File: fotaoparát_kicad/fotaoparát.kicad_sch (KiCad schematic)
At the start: 5 parts, among them IC1 W25Q256JVEIQ, J2 Micro_SD_Card_Det1, U2 CR2013-MI2120

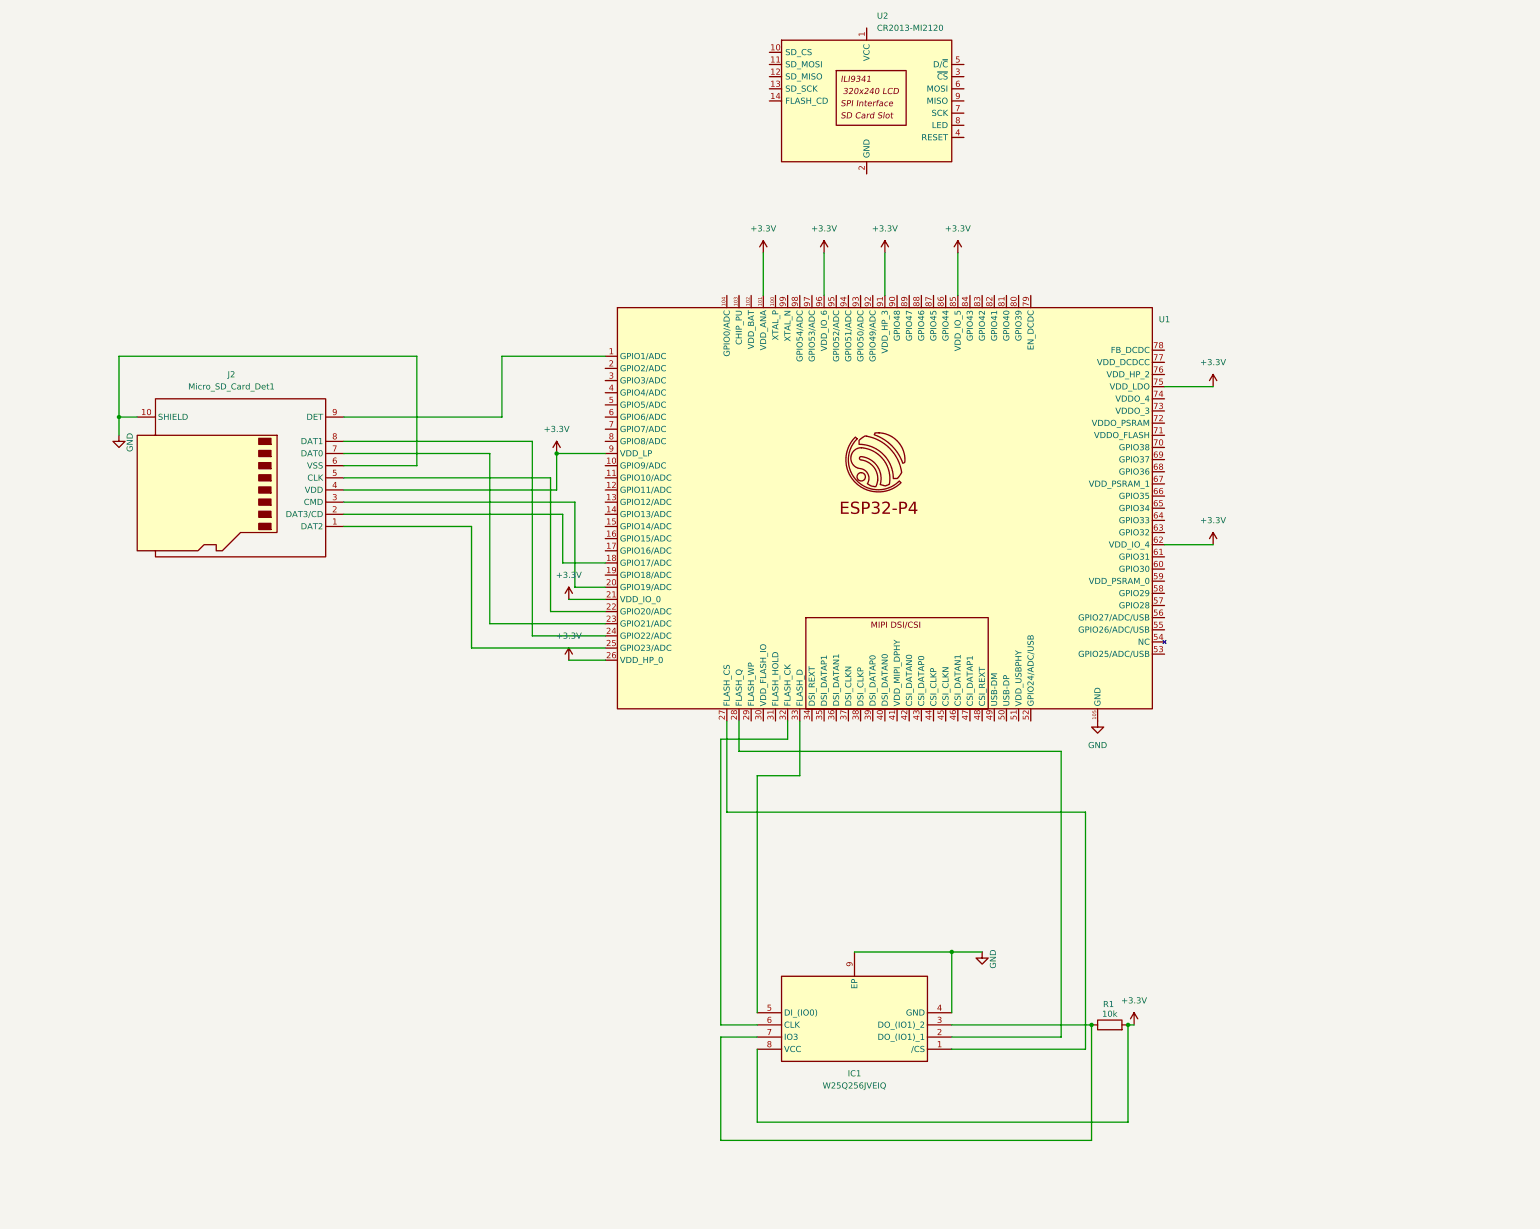
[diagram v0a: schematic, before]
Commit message: blablabla
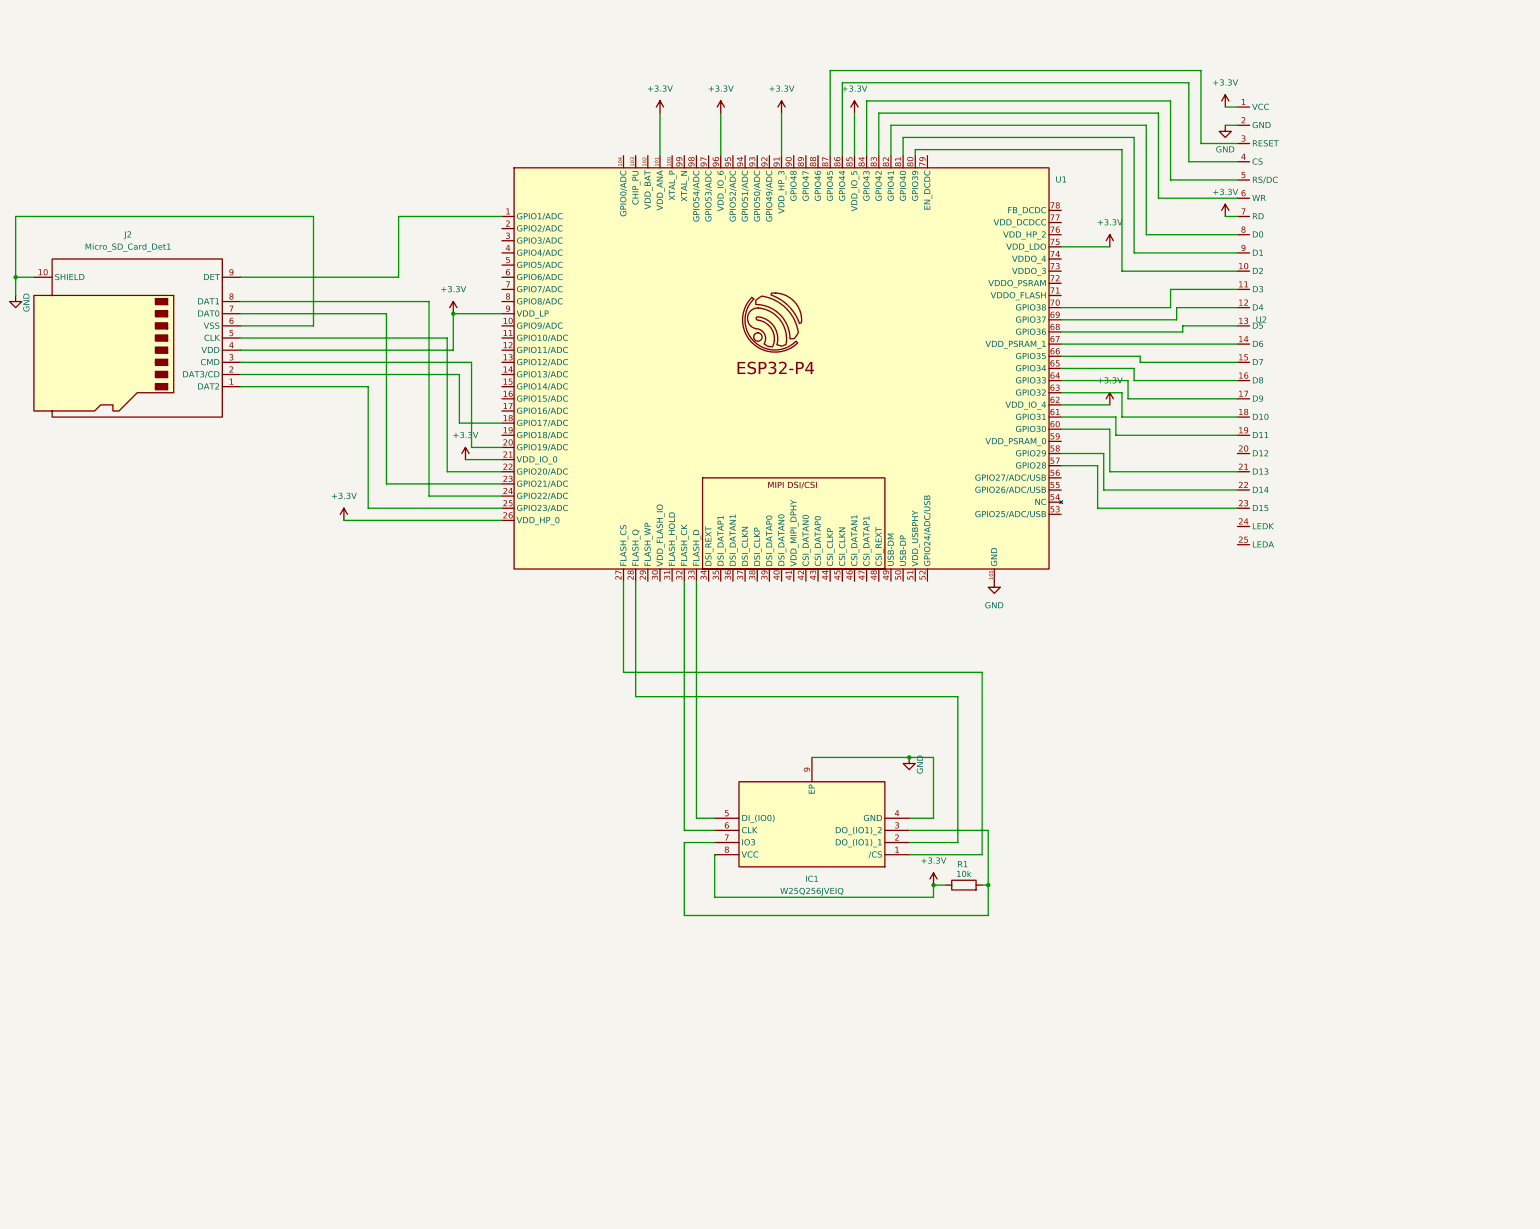
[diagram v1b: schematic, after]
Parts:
- removed U2: CR2013-MI2120, Display:CR2013-MI2120, symbol Driver_Display:CR2013-MI2120
- added U2: ~, symbol st_lib:ST7796s
- J2: footprint (none) -> Connector_Card:microSD_HC_Hirose_DM3D-SF
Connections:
- net +3.3V: now also R1.1, U2.1 (VCC), U2.7 (RD); no longer R1.2
- net GND: now also U2.2 (GND)
- net at U1.57 (GPIO28): now also U2.23 (D15)
- net at U1.58 (GPIO29): now also U2.22 (D14)
- net at U1.60 (GPIO30): now also U2.21 (D13)
- net at U1.61 (GPIO31): now also U2.19 (D11)
- net at U1.63 (GPIO32): now also U2.18 (D10)
- net at U1.64 (GPIO33): now also U2.17 (D9)
- net at U1.65 (GPIO34): now also U2.16 (D8)
- net at U1.66 (GPIO35): now also U2.15 (D7)
- net at U1.67 (VDD_PSRAM_1): now also U2.14 (D6)
- net at U1.68 (GPIO36): now also U2.13 (D5)
- net at U1.69 (GPIO37): now also U2.12 (D4)
- net at U1.70 (GPIO38): now also U2.11 (D3)
- net at U1.80 (GPIO39): now also U2.10 (D2)
- net at U1.81 (GPIO40): now also U2.9 (D1)
- net at U1.82 (GPIO41): now also U2.8 (D0)
- net at U1.83 (GPIO42): now also U2.6 (WR)
- net at U1.84 (GPIO43): now also U2.5 (RS/DC)
- net at U1.86 (GPIO44): now also U2.4 (CS)
- net at U1.87 (GPIO45): now also U2.3 (RESET)
- net at IC1.3 (DO_(IO1)_2), IC1.7 (IO3): now also R1.2; no longer R1.1
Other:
- moved on the sheet: IC1, J2, R1, U1

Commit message: nevim, neco tu vadi
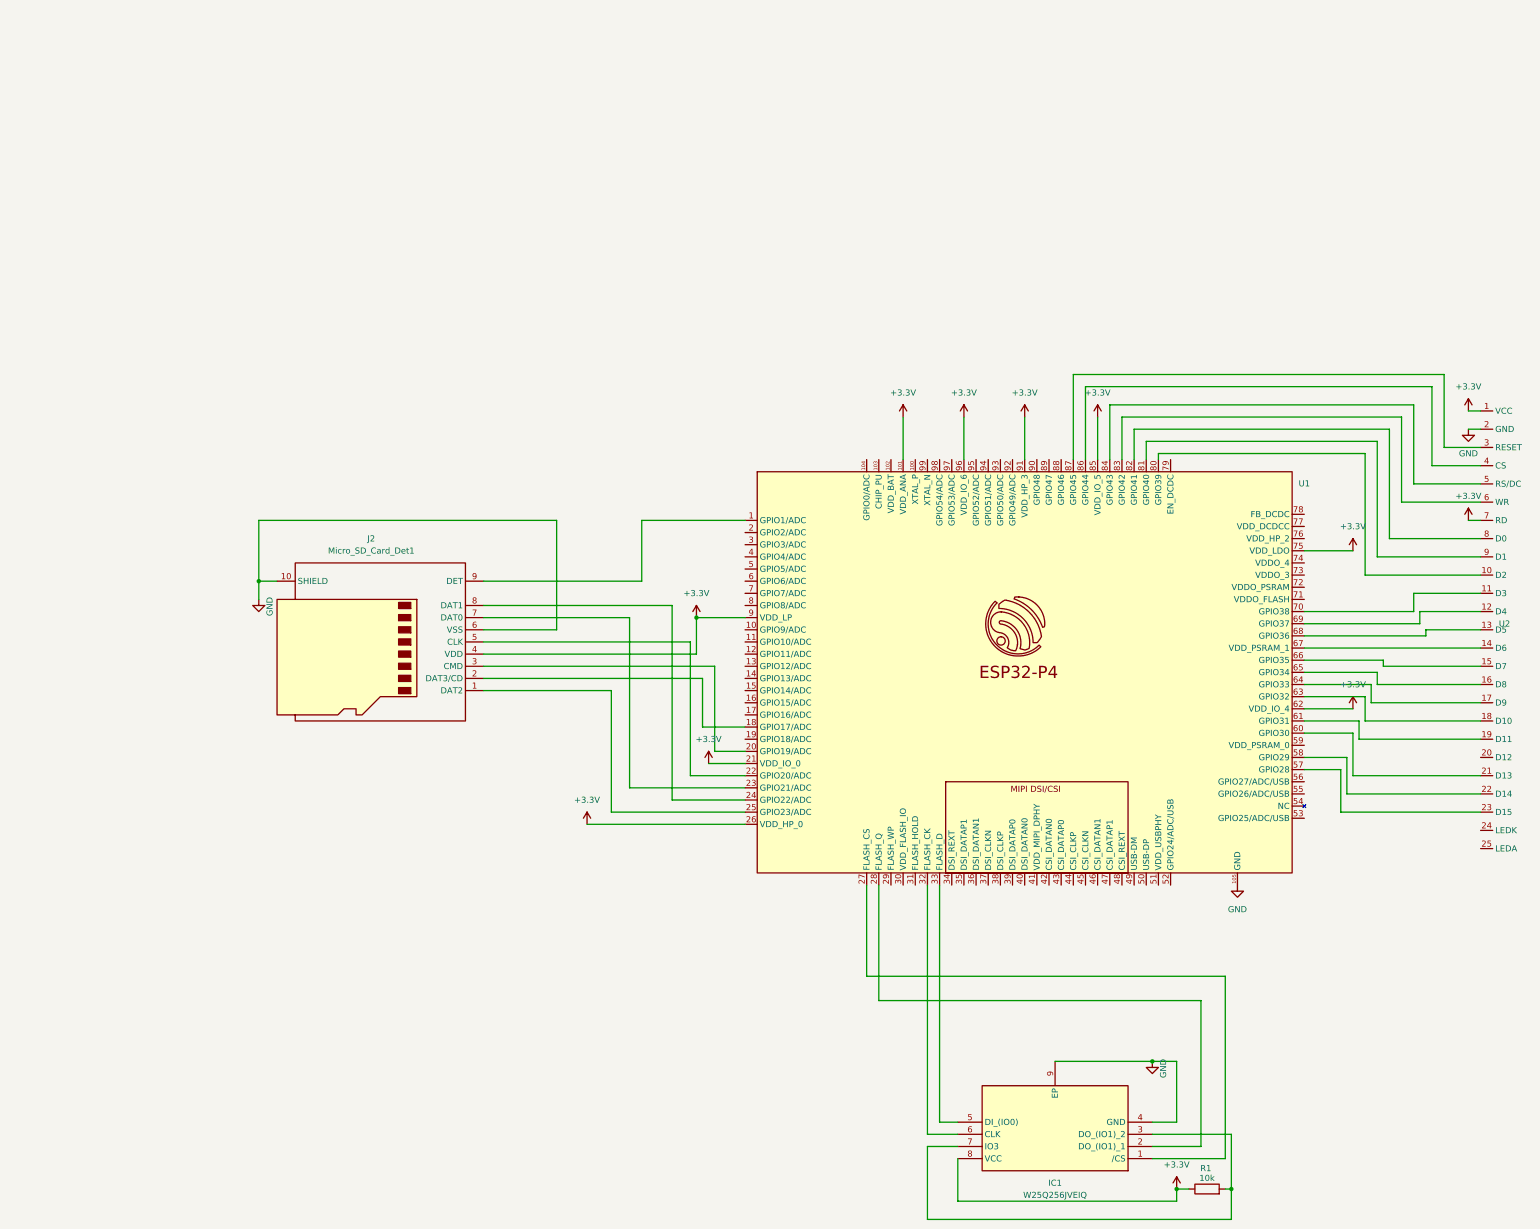
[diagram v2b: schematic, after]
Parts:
- U2: footprint (none) -> stlib:ST7796s_40PIN_0.8MM
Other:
- moved on the sheet: IC1, J2, R1, U1, U2
